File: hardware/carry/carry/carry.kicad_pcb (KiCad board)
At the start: 2 copper layers, 65 parts, among them J1 LEFT IN, J2 RIGHT IN, J3 LEFT OUT, J4 RIGHT OUT, J5 694106301002, J6 Conn_02x22_Odd_Even, J7 JST XH, U1 MCP6002-E/SN, U2 MCP6002-E/SN, U3 AZ1117CH2-5.0, U4 BU33SD5WG-TR, U5 BU33SD5WG-TR

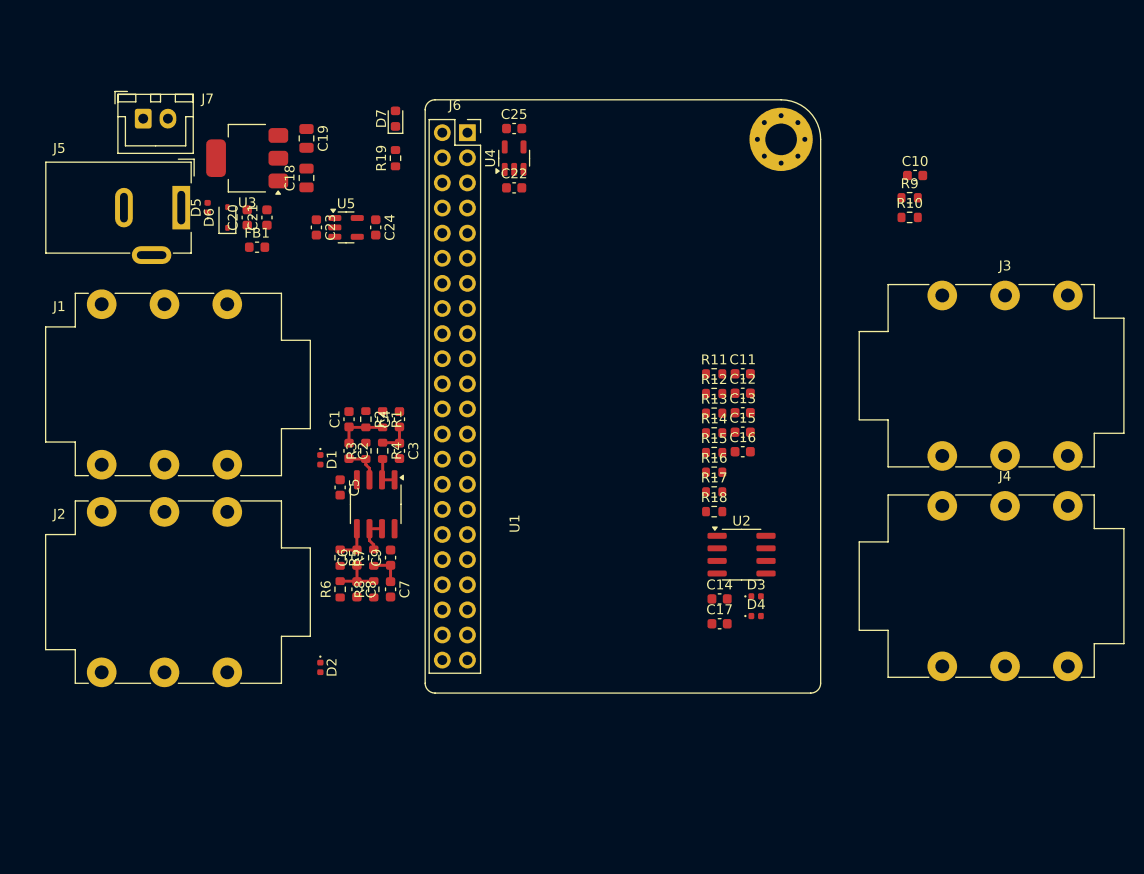
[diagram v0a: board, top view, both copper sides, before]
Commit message: routing carry board
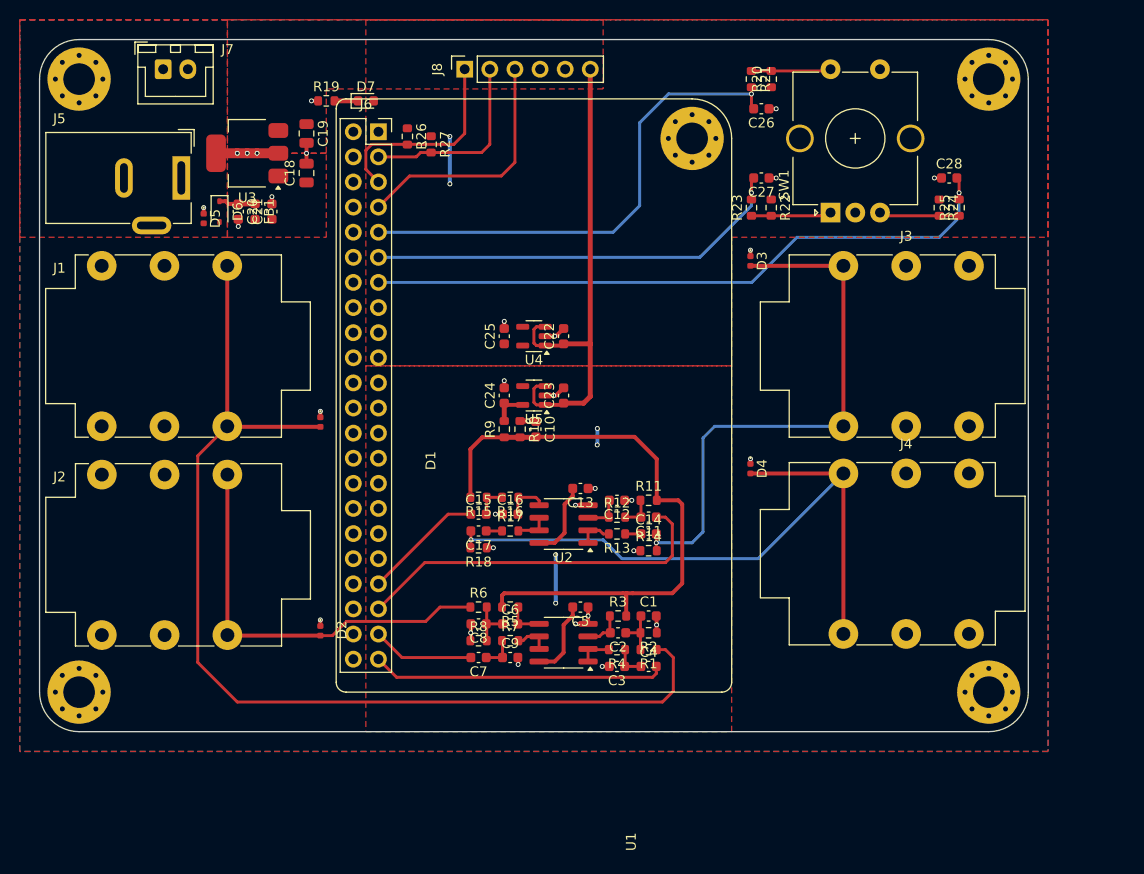
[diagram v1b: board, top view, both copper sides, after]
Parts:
- added C26: 100n, Capacitor_SMD:C_0603_1608Metric, F.Cu at (113.0, 37.0)
- added C27: 100n, Capacitor_SMD:C_0603_1608Metric, F.Cu at (113.0, 44.0)
- added C28: 100n, Capacitor_SMD:C_0603_1608Metric, F.Cu at (132.0, 44.0)
- added H2: MountingHole_Pad, MountingHole:MountingHole_3.2mm_M3_Pad_Via, F.Cu at (44.0, 34.0)
- added H3: MountingHole_Pad, MountingHole:MountingHole_3.2mm_M3_Pad_Via, F.Cu at (136.0, 34.0)
- added H4: MountingHole_Pad, MountingHole:MountingHole_3.2mm_M3_Pad_Via, F.Cu at (136.0, 96.0)
- added H5: MountingHole_Pad, MountingHole:MountingHole_3.2mm_M3_Pad_Via, F.Cu at (44.0, 96.0)
- added J8: Conn_01x06, Connector_PinSocket_2.54mm:PinSocket_1x06_P2.54mm_Vertical, F.Cu at (83.0, 33.0)
- added R20: 100k, Resistor_SMD:R_0603_1608Metric, F.Cu at (114.0, 34.0)
- added R21: 100k, Resistor_SMD:R_0603_1608Metric, F.Cu at (112.0, 34.0)
- added R22: 100k, Resistor_SMD:R_0603_1608Metric, F.Cu at (114.0, 47.0)
- added R23: 100k, Resistor_SMD:R_0603_1608Metric, F.Cu at (112.0, 47.0)
- added R24: 100k, Resistor_SMD:R_0603_1608Metric, F.Cu at (131.0, 47.0)
- added R25: 100k, Resistor_SMD:R_0603_1608Metric, F.Cu at (133.0, 47.0)
- added R26: 2.2k, Resistor_SMD:R_0603_1608Metric, F.Cu at (77.2, 39.8)
- added R27: 2.2k, Resistor_SMD:R_0603_1608Metric, F.Cu at (79.6, 40.6)
- added SW1: RotaryEncoder_Switch, Rotary_Encoder:RotaryEncoder_Alps_EC12E-Switch_Vertical_H20mm_CircularMountingHoles, F.Cu at (120.0, 47.5)
- moved R9 47.2 mm to (87.0, 69.4), turned to 90 degrees
- moved C10 46.1 mm to (90.2, 69.4), turned to -90 degrees
- moved R10 44.8 mm to (88.6, 69.4), turned to -90 degrees
- moved C1 36.3 mm to (101.6, 88.3), turned to 0 degrees
- moved R2 35.8 mm to (101.6, 90.0), turned to 180 degrees
- moved R1 35.6 mm to (101.6, 91.7), turned to 180 degrees
- moved C4 35.5 mm to (101.6, 93.4), turned to 0 degrees
- moved D3 33.9 mm to (111.9, 52.4), turned to -90 degrees
- moved C2 32.8 mm to (98.5, 90.0), turned to 180 degrees
- moved R4 31.1 mm to (98.4, 91.7), turned to 180 degrees
- moved C3 31.0 mm to (98.4, 93.4), turned to 180 degrees
- moved R3 30.5 mm to (98.5, 88.3), turned to 0 degrees
- moved C23 30.2 mm to (93.0, 66.0), turned to 90 degrees
- moved C15 28.0 mm to (84.4, 78.0)
- moved C5 27.1 mm to (94.7, 87.4), turned to 180 degrees
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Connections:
- J6 pad 11: /DSP SOM Slot/ADC3_IN2 -> /DSP SOM Slot/ENC_A
- J6 pad 13: /DSP SOM Slot/ADC3_IN3 -> /DSP SOM Slot/ENC_B
- J6 pad 3: /DSP SOM Slot/PB10 -> /DSP SOM Slot/OLED_SCL
- J6 pad 37: /Analog Back-End/CODEC_OUT_L -> /Analog Back-End/CODEC_OUT_R
- J6 pad 39: /Analog Back-End/CODEC_OUT_R -> /Analog Back-End/CODEC_OUT_L
- J6 pad 41: /Analog Front-End/CODEC_L_IN -> /Analog Front-End/CODEC_R_IN
- J6 pad 43: /Analog Front-End/CODEC_R_IN -> /Analog Front-End/CODEC_L_IN
- J6 pad 5: /DSP SOM Slot/PB11 -> /DSP SOM Slot/OLED_SDA
- J6 pad 7: /DSP SOM Slot/PD12 -> /DSP SOM Slot/OLED_RST
- J6 pad 9: /DSP SOM Slot/PD13 -> /DSP SOM Slot/ENC_PB
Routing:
- net Net-(D1-A2): track 0.00 -> 106.4 mm
- net Net-(D4-A2): track 0.00 -> 69.4 mm, vias 0 -> 1
- net /DSP SOM Slot/ENC_B: track 0.00 -> 66.2 mm, vias 0 -> 1
- net /Analog Back-End/VREF: track 0.00 -> 63.0 mm
- net Net-(D3-A2): track 0.00 -> 56.7 mm, vias 0 -> 1
- net /DSP SOM Slot/ENC_PB: track 0.00 -> 50.7 mm, vias 0 -> 1
- net +5V: track 0.00 -> 50.4 mm
- net /DSP SOM Slot/ENC_A: track 0.00 -> 43.5 mm, vias 0 -> 1
- net Net-(D2-A2): track 0.00 -> 42.0 mm
- net /Analog Back-End/CODEC_OUT_L: track 0.00 -> 37.1 mm
- net GND: track 0.00 -> 35.7 mm, vias 0 -> 32
- net /Analog Front-End/CODEC_L_IN: track 0.00 -> 29.7 mm
- net +3.3VA: track 0.00 -> 26.0 mm, vias 0 -> 4
- net /DSP SOM Slot/OLED_RST: track 0.00 -> 25.1 mm
- net /DSP SOM Slot/OLED_SDA: track 0.00 -> 20.9 mm
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- added copper zone on F.Cu, net +3.3V
- added copper zone on F.Cu, net +3.3VA
- added copper zone on F.Cu, net +5V
- added copper zone on F.Cu, net /Power Supply/9V_CONNECTOR
- added copper zone on F.Cu, net /Power Supply/9V_FILT
- added copper zone on B.Cu, net GND
- added copper zone on F.Cu, net GND
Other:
- board outline added: 100 x 70 mm
